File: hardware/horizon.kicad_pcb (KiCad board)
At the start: 4 copper layers, 95 x 56.2 mm, 39 parts, among them J1 Conn_01x02_Pin, J2 Conn_01x06_Pin, J3 USB_C_Receptacle_USB2.0_14P, J4 Conn_01x14_Pin, J5 Conn_01x02_Socket, J6 Conn_01x02_Pin, Q1 NPN, SW1 SW_Push, SW2 SW_Push, U1 ESP32-S3, U2 NCP1529A, U3 W25Q128JVS, U4 BQ24074RGT, U5 DRV2605LDGS, Y1 CDX-1293

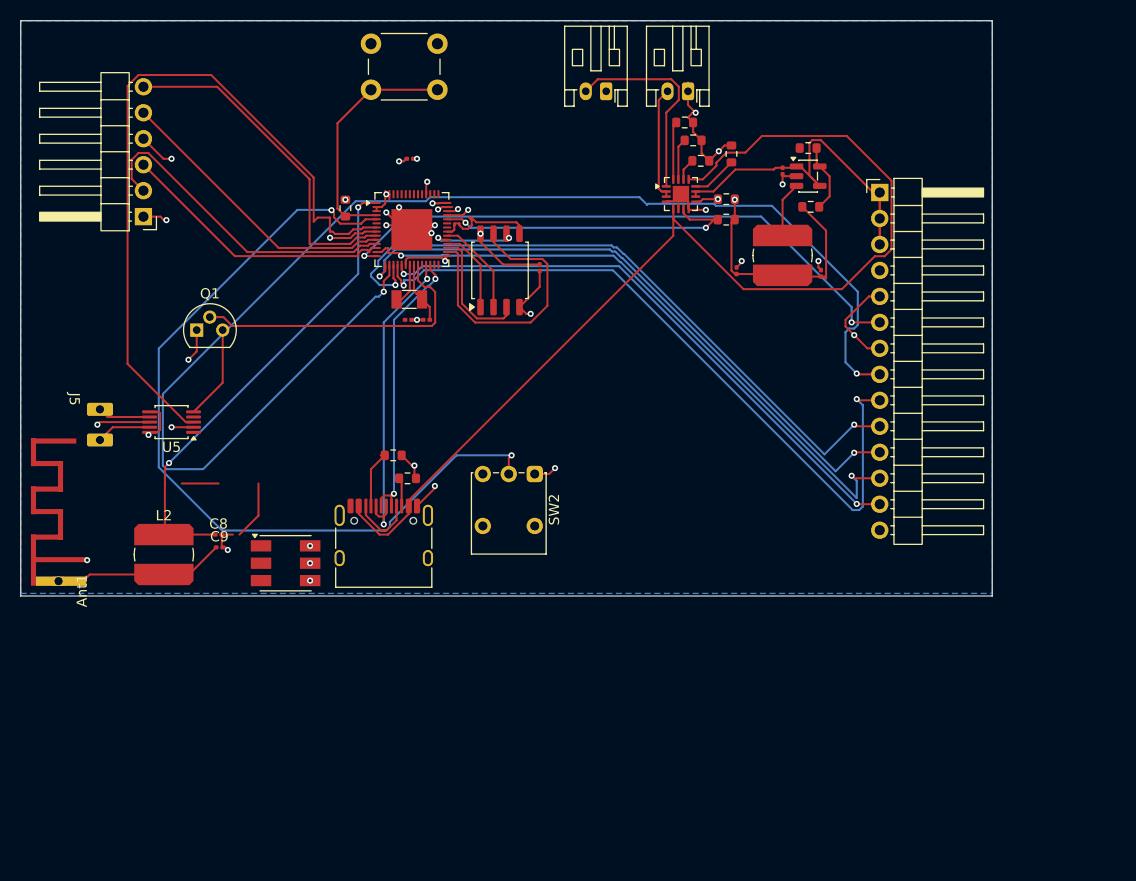
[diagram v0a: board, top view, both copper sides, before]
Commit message: Redoing pcb and fixed schem
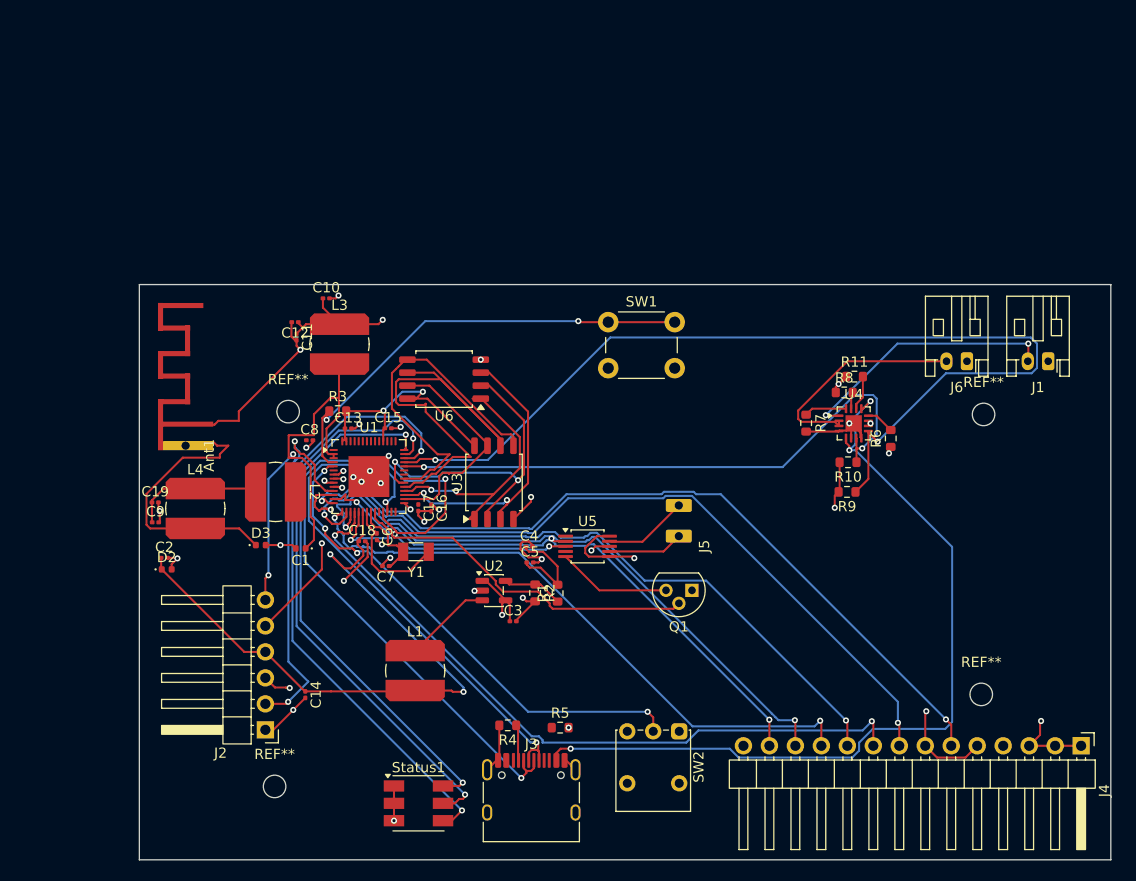
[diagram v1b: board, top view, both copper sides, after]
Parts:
- added C10: 0.1uF, Capacitor_SMD:C_0201_0603Metric, F.Cu at (119.9, 52.1)
- added C11: 1uF, Capacitor_SMD:C_0201_0603Metric, F.Cu at (117.0, 55.9)
- added C12: 1uF, Capacitor_SMD:C_0201_0603Metric, F.Cu at (116.8, 54.5)
- added C13: 1uF, Capacitor_SMD:C_0201_0603Metric, F.Cu at (122.0, 64.9)
- added C14: 10nF, Capacitor_SMD:C_0201_0603Metric, F.Cu at (117.8, 90.9)
- added C15: 0.1uF, Capacitor_SMD:C_0201_0603Metric, F.Cu at (125.9, 64.8)
- added C16: 1uF, Capacitor_SMD:C_0201_0603Metric, F.Cu at (130.2, 72.7)
- added C17: 0.1uF, Capacitor_SMD:C_0201_0603Metric, F.Cu at (128.9, 72.6)
- added C18: 0.1uF, Capacitor_SMD:C_0201_0603Metric, F.Cu at (123.4, 75.9)
- added C19: TBD, Capacitor_SMD:C_0201_0603Metric, F.Cu at (103.2, 72.1)
- added D2: D_TVS, Diode_SMD:D_0402_1005Metric, F.Cu at (104.3, 78.7)
- added D3: D_TVS, Diode_SMD:D_0402_1005Metric, F.Cu at (113.5, 76.3)
- added L3: L, Inductor_SMD:L_Bourns_SDR0604, F.Cu at (121.2, 56.6)
- added L4: TBD, Inductor_SMD:L_Bourns_SDR0604, F.Cu at (107.1, 72.7)
- added REF**: MountingHole_2.2mm_M2, MountingHole:MountingHole_2.2mm_M2, F.Cu at (114.8, 99.9)
- added REF**: MountingHole_2.2mm_M2, MountingHole:MountingHole_2.2mm_M2, F.Cu at (183.9, 90.9)
- added REF**: MountingHole_2.2mm_M2, MountingHole:MountingHole_2.2mm_M2, F.Cu at (116.2, 63.2)
- added REF**: MountingHole_2.2mm_M2, MountingHole:MountingHole_2.2mm_M2, F.Cu at (184.2, 63.5)
- added U6: ESP-PSRAM64H, Package_SO:SOIC-8_5.3x5.3mm_P1.27mm, F.Cu at (131.4, 60.0)
- C1: value 100nF -> 0.1uF; footprint Capacitor_SMD:C_0201_0603Metric -> Diode_SMD:D_0402_1005Metric
- C2: value 100nF -> 10uF
- C8, C9: value 3P3 -> TBD
- L2: value 2n2 -> TBD
- moved J5 64.2 mm to (157.3, 76.4), turned to 90 degrees
- moved J4 57.6 mm to (193.7, 95.9), turned to -90 degrees
- moved Q1 54.7 mm to (155.6, 80.7), turned to 180 degrees
- moved L1 54.2 mm to (128.6, 88.5)
- moved J2 51.6 mm to (113.9, 94.3)
- moved C3 51.3 mm to (138.2, 83.7), turned to 0 degrees
- moved R2 51.0 mm to (140.3, 81.0), turned to -90 degrees
- moved U2 50.9 mm to (136.3, 80.7)
- moved J1 50.6 mm to (190.5, 58.3)
- moved C2 46.4 mm to (104.0, 77.5), turned to 0 degrees
- moved R1 45.2 mm to (142.5, 81.0), turned to 90 degrees
- moved U5 42.5 mm to (145.4, 76.4), turned to 0 degrees
- moved C1 39.6 mm to (117.4, 76.6), turned to 180 degrees
- moved C4 39.1 mm to (139.7, 76.4), turned to 0 degrees
- moved J6 38.0 mm to (182.5, 58.3)
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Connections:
- Ant1 pad 1: Net-(Ant1-Pad1) -> Net-(D3-A1)
- C1 pad 1: +3.3V -> Net-(C1-Pad1)
- C2 pad 1: +3.3V -> VDD_SPI
- C4 pad 1: +3.3V -> VDD_SPI
- C5 pad 1: +3.3V -> VDD_SPI
- C9 pad 1: Net-(Ant1-Pad1) -> Net-(C19-Pad1)
- J2 pad 4: +3.3V -> VDD_SPI
- L1 pad 2: +3.3V -> VDD_SPI
- L2 pad 2: Net-(Ant1-Pad1) -> Net-(C19-Pad1)
- R1 pad 2: +3.3V -> VDD_SPI
- R10 pad 2: +3.3V -> VDD_SPI
- R3 pad 2: +3.3V -> VDD_SPI
- R9 pad 2: +3.3V -> VDD_SPI
- SW2 pad 1: +3.3V -> VDD_SPI
- U1 pad 2: +3.3V -> Net-(C1-Pad1)
- U1 pad 20: +3.3V -> VDD_SPI
- U1 pad 29: +3.3V -> VDD_SPI
- U1 pad 3: +3.3V -> Net-(C1-Pad1)
- U1 pad 46: +3.3V -> VDD_SPI
- U1 pad 55: +3.3V -> VDD_SPI
- U1 pad 56: +3.3V -> VDD_SPI
- U3 pad 8: +3.3V -> VDD_SPI
- U5 pad 10: +3.3V -> VDD_SPI
- U5 pad 6: +3.3V -> VDD_SPI
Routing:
- net VDD_SPI: track 0.00 -> 244.5 mm, vias 0 -> 9
- net +5V: track 37.9 -> 108.8 mm, vias 0 -> 3
- net CHG: track 30.0 -> 96.1 mm
- net SPI_MOSI: track 130.1 -> 76.9 mm
- net +3.3V: track 52.7 -> 0.00 mm, vias 10 -> 0
- net Net-(U1-LNA_IN): track 46.9 -> 0.00 mm, vias 2 -> 0
- net HAPTIC_SDA: track 71.1 -> 28.0 mm, vias 0 -> 3
- net USB_D-: track 30.7 -> 68.4 mm
- net QSPI_CLK: track 8.63 -> 45.6 mm, vias 2 -> 0
- net Net-(U1-GPIO0): track 81.9 -> 49.3 mm, vias 2 -> 4
- net Net-(C1-Pad1): track 0.00 -> 31.1 mm
- net GND: track 74.1 -> 101.0 mm, vias 24 -> 30
- net Net-(D3-A1): track 0.00 -> 26.8 mm
- net PGOOD: track 31.2 -> 57.7 mm
- net USB_D+: track 27.6 -> 52.5 mm
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- added copper zone on In1.Cu, net GND
- removed copper zone on In2.Cu, net +3.3V
- removed copper zone on B.Cu, net GND
